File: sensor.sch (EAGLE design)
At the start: 60 parts, among them CN3 15PIN 0.5MM, U1 TCD2565BFG, U10 LT1806, U11 SN74LVC2G17, U12 SN74LVC2G17, U13 SN74LVC2G17, U14 SN74LVC2G17, U15 SN74LVC2G17, U19 AD5258BRMZ1-R7, U20 SN74LVC2G17, U21 AD5258BRMZ1-R7, U22 AD5258BRMZ1-R7, U3 ADS7056, U6 LT1806, U7 ADS7056, U8 LT1806, U9 ADS7056

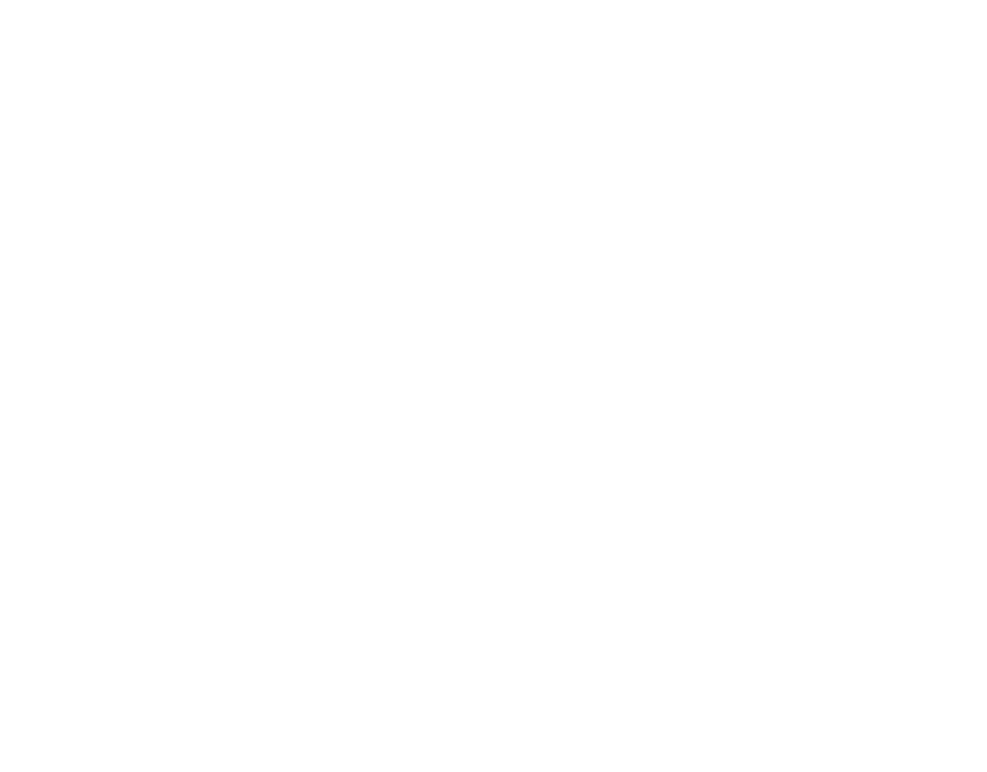
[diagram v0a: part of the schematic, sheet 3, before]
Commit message: Controller nearly done
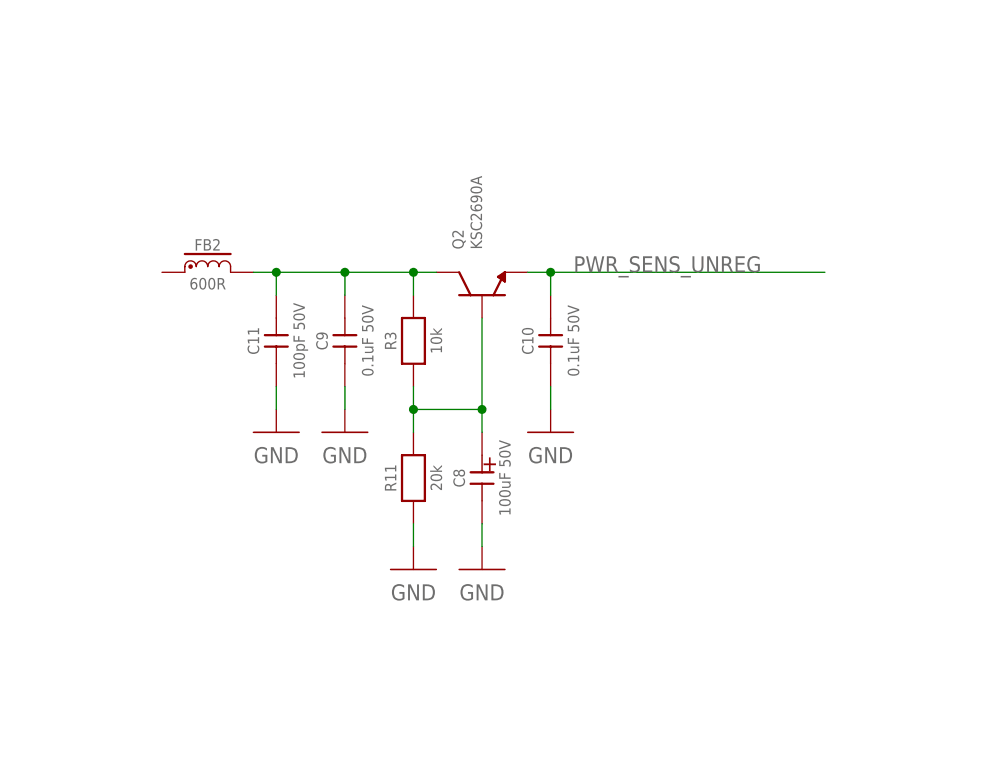
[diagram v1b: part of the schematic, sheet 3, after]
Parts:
- added C10, C9: 0.1uF 50V, c_0603:06035C104JAT2A
- added C11: 100pF 50V, c_0603:06035A101J4T4A
- added C8: 100uF 50V, CAPACITORS:107CKR050M
- added FB2: 600R, INDUCTORS:742792651
- added Q2: KSC2690A, TRANSISTORs:KSC2690AV
- added R11: 20k, r_0603:CRCW060320K0FKEA
- added R3: 10k, r_0603:CRCW060310K0FKTA
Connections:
- new net N$3: C11.2, C9.2, FB2.2, Q2.C, R3.2
- new net N$4: C8.A, Q2.B, R11.2, R3.1
- new net PWR_SENS_UNREG: C10.2, Q2.E
- net GND: now also C10.1, C11.1, C8.K, C9.1, R11.1
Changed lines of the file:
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@@
 <part name="GND76" library="NETS" deviceset="GND" device=""/>
 <part name="CN3" library="CONNECTORs" deviceset="SFV15R-1STE1HLF" device="" value="15PIN 0.5MM"/>
+<part name="Q2" library="TRANSISTORs" deviceset="KSC2690A" device="V" value="KSC2690A"/>
+<part name="R3" library="r_0603" deviceset="CRCW060310K0FKTA" device="" value="10k"/>
+<part name="R11" library="r_0603" deviceset="CRCW060320K0FKEA" device="" value="20k"/>
+<part name="C8" library="CAPACITORS" deviceset="107CKR050M" device="" value="100uF 50V"/>
+<part name="GND4" library="NETS" deviceset="GND" device=""/>
+<part name="GND5" library="NETS" deviceset="GND" device=""/>
+<part name="C9" library="c_0603" deviceset="06035C104JAT2A" device="" value="0.1uF 50V"/>
+<part name="C10" library="c_0603" deviceset="06035C104JAT2A" device="" value="0.1uF 50V"/>
+<part name="C11" library="c_0603" deviceset="06035A101J4T4A" device="" value="100pF 50V"/>
+<part name="FB2" library="INDUCTORS" deviceset="742792651" device="" value="600R"/>
+<part name="GND6" library="NETS" deviceset="GND" device=""/>
+<part name="GND7" library="NETS" deviceset="GND" device=""/>
+<part name="GND8" library="NETS" deviceset="GND" device=""/>
 </parts>
 <sheets>
@@
 </plain>
 <instances>
+<instance part="Q2" gate="G$1" x="-93.98" y="203.2" smashed="yes" rot="R90">
+<attribute name="NAME" x="-96.012" y="205.74" size="1.27" layer="95" rot="R90"/>
+<attribute name="VALUE" x="-93.98" y="205.74" size="1.27" layer="96" rot="R90"/>
+</instance>
+<instance part="R3" gate="G$1" x="-101.6" y="195.58" smashed="yes" rot="R90">
+<attribute name="NAME" x="-104.14" y="195.58" size="1.27" layer="95" rot="R90" align="center"/>
+<attribute name="VALUE" x="-99.06" y="195.58" size="1.27" layer="96" rot="R90" align="center"/>
+</instance>
+<instance part="R11" gate="G$1" x="-101.6" y="180.34" smashed="yes" rot="R90">
+<attribute name="NAME" x="-104.14" y="180.34" size="1.27" layer="95" rot="R90" align="center"/>
+<attribute name="VALUE" x="-99.06" y="180.34" size="1.27" layer="96" rot="R90" align="center"/>
+</instance>
+<instance part="C8" gate="G$1" x="-93.98" y="180.34" smashed="yes" rot="R90">
+<attribute name="NAME" x="-96.52" y="180.34" size="1.27" layer="95" rot="R90" align="center"/>
+<attribute name="VALUE" x="-91.44" y="180.34" size="1.27" layer="96" rot="R90" align="center"/>
+</instance>
+<instance part="GND4" gate="G$1" x="-101.6" y="170.18" smashed="yes">
+<attribute name="VALUE" x="-101.6" y="167.64" size="1.778" layer="96" align="center"/>
+</instance>
+<instance part="GND5" gate="G$1" x="-93.98" y="170.18" smashed="yes">
+<attribute name="VALUE" x="-93.98" y="167.64" size="1.778" layer="96" align="center"/>
+</instance>
+<instance part="C9" gate="G$1" x="-109.22" y="195.58" smashed="yes" rot="R90">
+<attribute name="NAME" x="-111.76" y="195.58" size="1.27" layer="95" rot="R90" align="center"/>
+<attribute name="VALUE" x="-106.68" y="195.58" size="1.27" layer="96" rot="R90" align="center"/>
+</instance>
+<instance part="C10" gate="G$1" x="-86.36" y="195.58" smashed="yes" rot="R90">
+<attribute name="NAME" x="-88.9" y="195.58" size="1.27" layer="95" rot="R90" align="center"/>
+<attribute name="VALUE" x="-83.82" y="195.58" size="1.27" layer="96" rot="R90" align="center"/>
+</instance>
+<instance part="C11" gate="G$1" x="-116.84" y="195.58" smashed="yes" rot="R90">
+<attribute name="NAME" x="-119.38" y="195.58" size="1.27" layer="95" rot="R90" align="center"/>
+<attribute name="VALUE" x="-114.3" y="195.58" size="1.27" layer="96" rot="R90" align="center"/>
+</instance>
+<instance part="FB2" gate="G$1" x="-124.46" y="203.2" smashed="yes">
+<attribute name="NAME" x="-124.46" y="206.248" size="1.27" layer="95" align="center"/>
+<attribute name="VALUE" x="-124.46" y="201.93" size="1.27" layer="96" align="center"/>
+</instance>
+<instance part="GND6" gate="G$1" x="-109.22" y="185.42" smashed="yes">
+<attribute name="VALUE" x="-109.22" y="182.88" size="1.778" layer="96" align="center"/>
+</instance>
+<instance part="GND7" gate="G$1" x="-116.84" y="185.42" smashed="yes">
+<attribute name="VALUE" x="-116.84" y="182.88" size="1.778" layer="96" align="center"/>
+</instance>
+<instance part="GND8" gate="G$1" x="-86.36" y="185.42" smashed="yes">
+<attribute name="VALUE" x="-86.36" y="182.88" size="1.778" layer="96" align="center"/>
+</instance>
 </instances>
 <busses>
 </busses>
 <nets>
+<net name="GND" class="0">
+<segment>
+<pinref part="R11" gate="G$1" pin="1"/>
+<pinref part="GND4" gate="G$1" pin="GND"/>
+<wire x1="-101.6" y1="172.72" x2="-101.6" y2="175.26" width="0.1524" layer="91"/>
+</segment>
+<segment>
+<pinref part="C8" gate="G$1" pin="K"/>
+<pinref part="GND5" gate="G$1" pin="GND"/>
+<wire x1="-93.98" y1="172.72" x2="-93.98" y2="175.26" width="0.1524" layer="91"/>
+</segment>
+<segment>
+<pinref part="C9" gate="G$1" pin="1"/>
+<pinref part="GND6" gate="G$1" pin="GND"/>
+<wire x1="-109.22" y1="187.96" x2="-109.22" y2="190.5" width="0.1524" layer="91"/>
+</segment>
+<segment>
+<pinref part="C11" gate="G$1" pin="1"/>
+<pinref part="GND7" gate="G$1" pin="GND"/>
+<wire x1="-116.84" y1="187.96" x2="-116.84" y2="190.5" width="0.1524" layer="91"/>
+</segment>
+<segment>
+<pinref part="C10" gate="G$1" pin="1"/>
+<pinref part="GND8" gate="G$1" pin="GND"/>
+<wire x1="-86.36" y1="187.96" x2="-86.36" y2="190.5" width="0.1524" layer="91"/>
+</segment>
+</net>
+<net name="N$3" class="0">
+<segment>
+<pinref part="Q2" gate="G$1" pin="C"/>
+<pinref part="R3" gate="G$1" pin="2"/>
+<wire x1="-116.84" y1="203.2" x2="-109.22" y2="203.2" width="0.1524" layer="91"/>
+<wire x1="-109.22" y1="203.2" x2="-101.6" y2="203.2" width="0.1524" layer="91"/>
+<wire x1="-101.6" y1="203.2" x2="-99.06" y2="203.2" width="0.1524" layer="91"/>
+<wire x1="-101.6" y1="200.66" x2="-101.6" y2="203.2" width="0.1524" layer="91"/>
+<junction x="-101.6" y="203.2"/>
+<pinref part="C9" gate="G$1" pin="2"/>
+<wire x1="-109.22" y1="200.66" x2="-109.22" y2="203.2" width="0.1524" layer="91"/>
+<junction x="-109.22" y="203.2"/>
+<pinref part="C11" gate="G$1" pin="2"/>
+<wire x1="-116.84" y1="200.66" x2="-116.84" y2="203.2" width="0.1524" layer="91"/>
+<junction x="-116.84" y="203.2"/>
+<wire x1="-119.38" y1="203.2" x2="-116.84" y2="203.2" width="0.1524" layer="91"/>
+<pinref part="FB2" gate="G$1" pin="2"/>
+</segment>
+</net>
+<net name="N$4" class="0">
+<segment>
+<pinref part="R3" gate="G$1" pin="1"/>
+<pinref part="R11" gate="G$1" pin="2"/>
+<wire x1="-101.6" y1="185.42" x2="-101.6" y2="187.96" width="0.1524" layer="91"/>
+<pinref part="Q2" gate="G$1" pin="B"/>
+<wire x1="-101.6" y1="187.96" x2="-101.6" y2="190.5" width="0.1524" layer="91"/>
+<wire x1="-93.98" y1="198.12" x2="-93.98" y2="187.96" width="0.1524" layer="91"/>
+<wire x1="-93.98" y1="187.96" x2="-101.6" y2="187.96" width="0.1524" layer="91"/>
+<junction x="-101.6" y="187.96"/>
+<pinref part="C8" gate="G$1" pin="A"/>
+<wire x1="-93.98" y1="185.42" x2="-93.98" y2="187.96" width="0.1524" layer="91"/>
+<junction x="-93.98" y="187.96"/>
+</segment>
+</net>
+<net name="PWR_SENS_UNREG" class="0">
+<segment>
+<pinref part="Q2" gate="G$1" pin="E"/>
+<wire x1="-88.9" y1="203.2" x2="-86.36" y2="203.2" width="0.1524" layer="91"/>
+<pinref part="C10" gate="G$1" pin="2"/>
+<wire x1="-86.36" y1="203.2" x2="-55.88" y2="203.2" width="0.1524" layer="91"/>
+<wire x1="-86.36" y1="200.66" x2="-86.36" y2="203.2" width="0.1524" layer="91"/>
+<junction x="-86.36" y="203.2"/>
+<label x="-83.82" y="203.2" size="1.778" layer="95"/>
+</segment>
+</net>
 </nets>
 </sheet>
